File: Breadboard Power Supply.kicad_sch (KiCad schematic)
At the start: 15 parts, among them J1 Conn_01x02, J2 Conn_01x02, J3 Conn_01x03, J4 Screw_Terminal_01x02, J5 Barrel_Jack, U1 LM7805_TO220, U2 LM317_TO-220

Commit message: footprints
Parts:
- C1, C2, C3: footprint (none) -> Capacitor_THT:C_Disc_D3.0mm_W1.6mm_P2.50mm
- D1: footprint (none) -> LED_THT:LED_D5.0mm
- J1, J2: footprint (none) -> Connector_PinHeader_2.54mm:PinHeader_1x02_P2.54mm_Vertical
- J3: footprint (none) -> Connector_PinHeader_2.54mm:PinHeader_1x03_P2.54mm_Vertical
- J4: footprint (none) -> TerminalBlock:TerminalBlock_bornier-2_P5.08mm
- J5: footprint (none) -> Connector_BarrelJack:BarrelJack_SwitchcraftConxall_RAPC10U_Horizontal
- R1, R2, R3: footprint (none) -> PCM_Resistor_THT_AKL:R_Axial_DIN0204_L3.6mm_D1.6mm_P7.62mm_Horizontal
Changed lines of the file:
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@@
 			)
 		)
-		(property "Footprint" ""
+		(property "Footprint" "Capacitor_THT:C_Disc_D3.0mm_W1.6mm_P2.50mm"
 			(at 87.3252 66.04 0)
 			(effects
@@
 			)
 		)
-		(property "Footprint" ""
+		(property "Footprint" "PCM_Resistor_THT_AKL:R_Axial_DIN0204_L3.6mm_D1.6mm_P7.62mm_Horizontal"
 			(at 66.04 55.118 90)
 			(effects
@@
 			)
 		)
-		(property "Footprint" ""
+		(property "Footprint" "LED_THT:LED_D5.0mm"
 			(at 66.04 40.64 0)
 			(effects
@@
 			)
 		)
-		(property "Footprint" ""
+		(property "Footprint" "Capacitor_THT:C_Disc_D3.0mm_W1.6mm_P2.50mm"
 			(at 67.0052 66.04 0)
 			(effects
@@
 			)
 		)
-		(property "Footprint" ""
+		(property "Footprint" "Connector_PinHeader_2.54mm:PinHeader_1x02_P2.54mm_Vertical"
 			(at 66.04 72.39 0)
 			(effects
@@
 			)
 		)
-		(property "Footprint" ""
+		(property "Footprint" "TerminalBlock:TerminalBlock_bornier-2_P5.08mm"
 			(at 90.17 82.55 0)
 			(effects
@@
 			)
 		)
-		(property "Footprint" ""
+		(property "Footprint" "PCM_Resistor_THT_AKL:R_Axial_DIN0204_L3.6mm_D1.6mm_P7.62mm_Horizontal"
 			(at 86.36 55.118 90)
 			(effects
@@
 			)
 		)
-		(property "Footprint" ""
+		(property "Footprint" "PCM_Resistor_THT_AKL:R_Axial_DIN0204_L3.6mm_D1.6mm_P7.62mm_Horizontal"
 			(at 76.2 55.118 90)
 			(effects
@@
 			)
 		)
-		(property "Footprint" ""
+		(property "Footprint" "Connector_BarrelJack:BarrelJack_SwitchcraftConxall_RAPC10U_Horizontal"
 			(at 67.31 26.416 0)
 			(effects
@@
 			)
 		)
-		(property "Footprint" ""
+		(property "Footprint" "Connector_PinHeader_2.54mm:PinHeader_1x02_P2.54mm_Vertical"
 			(at 86.36 72.39 0)
 			(effects
@@
 			)
 		)
-		(property "Footprint" ""
+		(property "Footprint" "Connector_PinHeader_2.54mm:PinHeader_1x03_P2.54mm_Vertical"
 			(at 67.31 83.82 0)
 			(effects
@@
 			)
 		)
-		(property "Footprint" ""
+		(property "Footprint" "Capacitor_THT:C_Disc_D3.0mm_W1.6mm_P2.50mm"
 			(at 77.1652 66.04 0)
 			(effects

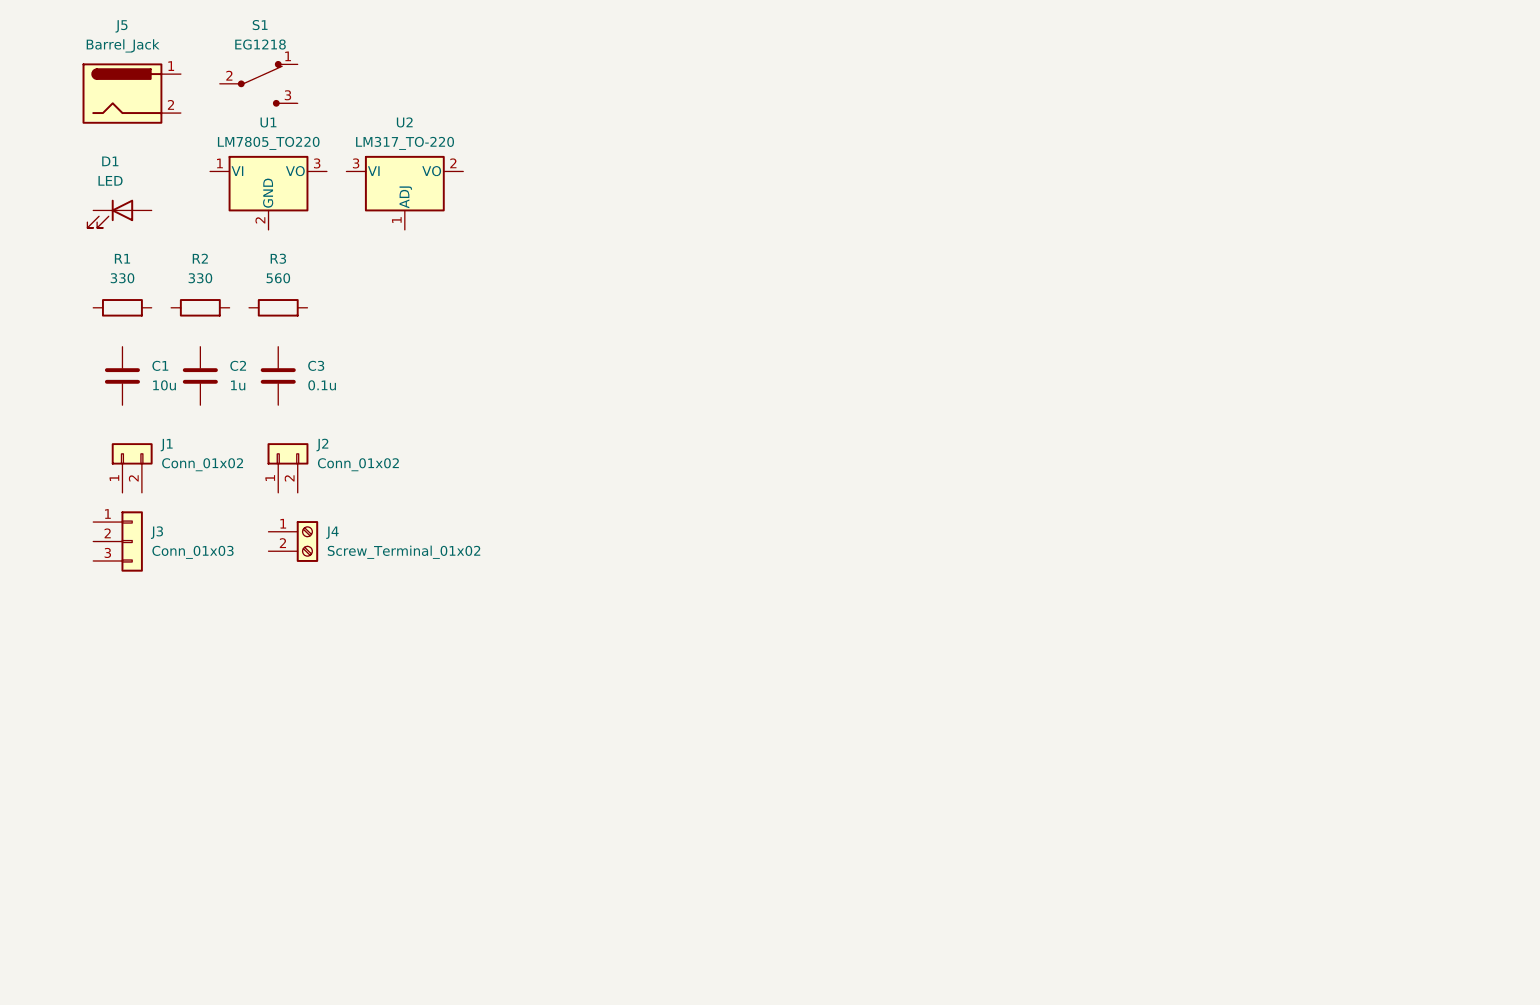
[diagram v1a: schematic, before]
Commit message: schematic + placing
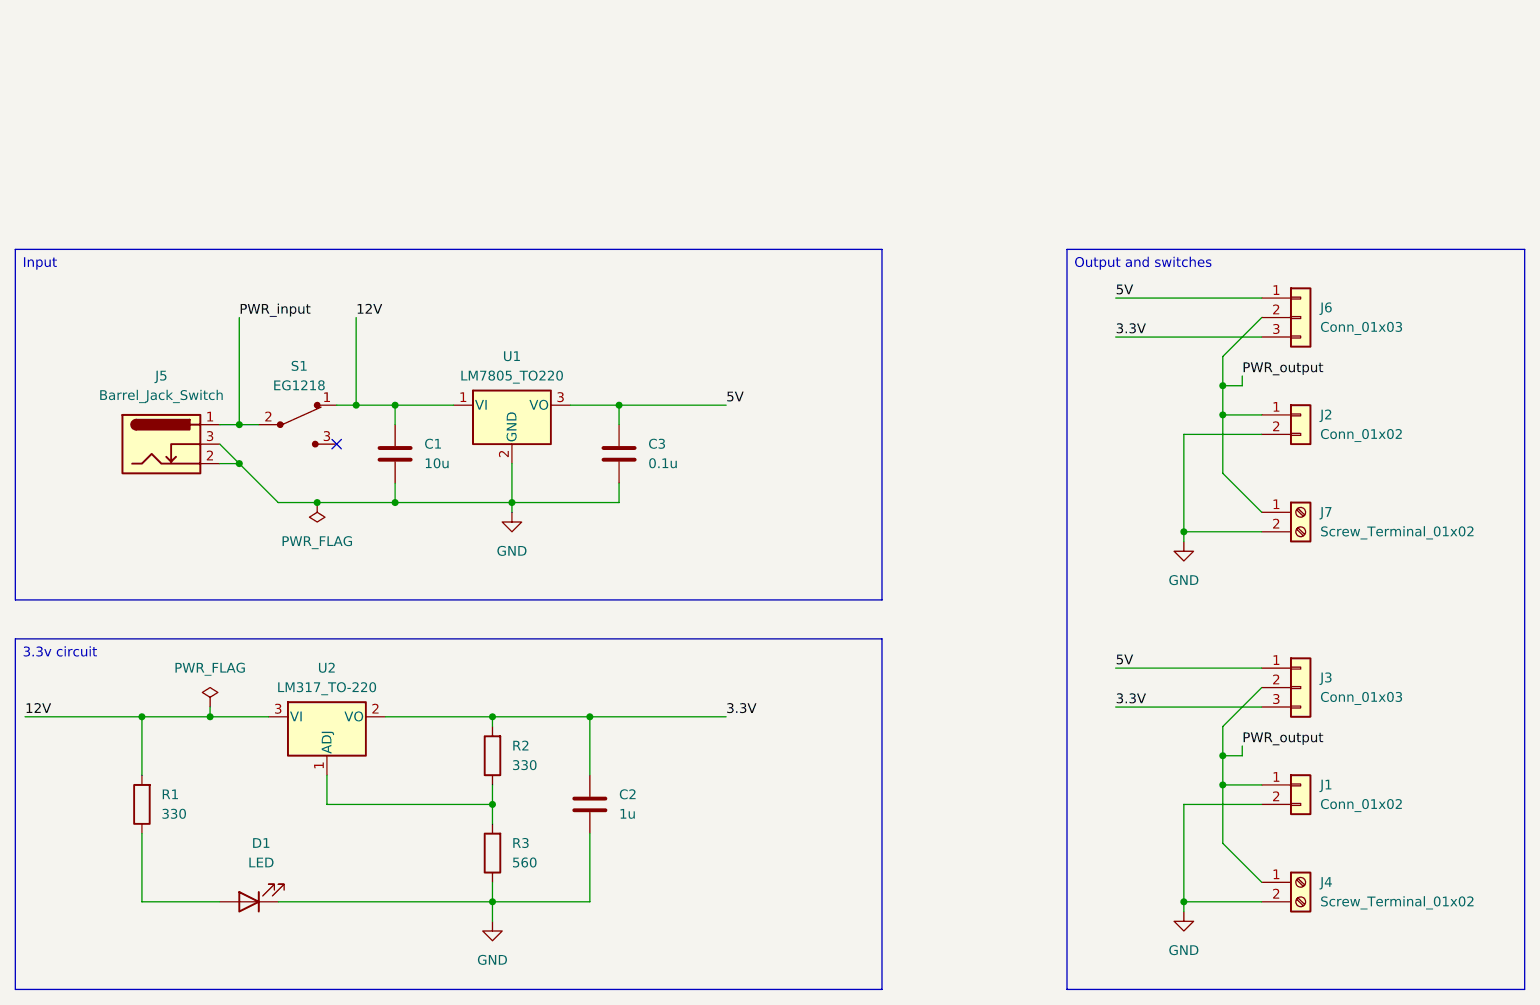
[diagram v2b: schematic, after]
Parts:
- removed J5: Barrel_Jack, Connector_BarrelJack:BarrelJack_SwitchcraftConxall_RAPC10U_Horizontal, symbol Connector:Barrel_Jack
- added J5: Barrel_Jack_Switch, Connector_BarrelJack:BarrelJack_Horizontal, symbol Connector:Barrel_Jack_Switch
- added J6: Conn_01x03, Connector_PinHeader_2.54mm:PinHeader_1x03_P2.54mm_Vertical, symbol Connector_Generic:Conn_01x03
- added J7: Screw_Terminal_01x02, TerminalBlock:TerminalBlock_bornier-2_P5.08mm, symbol Connector:Screw_Terminal_01x02
- D1: footprint LED_THT:LED_D5.0mm -> (none)
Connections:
- net 12V: now reaches S1.1
- net 12V: now also C1.1, R1.2, U1.1 (VI), U2.3 (VI)
- net PWR_input: now reaches S1.2
- net PWR_input: now also J5.1
- net 5V: now reaches C3.1
- net 5V: now also J3.1 (Pin_1), U1.3 (VO), J6.1 (Pin_1)
- net GND: now reaches C3.2
- net GND: now also C1.2, C2.2, D1.1 (K), J1.2 (Pin_2), J2.2 (Pin_2), J4.2 (Pin_2), R3.1, U1.2 (GND), J5.2, J5.3, J7.2 (Pin_2)
- net at R1.1: now also D1.2 (A)
- net PWR_output: now reaches J1.1 (Pin_1)
- net PWR_output: now also J2.1 (Pin_1), J3.2 (Pin_2), J4.1 (Pin_1), J6.2 (Pin_2), J7.1 (Pin_1)
- net at U2.1 (ADJ): now also R2.1, R3.2
- net 3.3V: now reaches U2.2 (VO)
- net 3.3V: now also C2.1, J3.3 (Pin_3), R2.2, J6.3 (Pin_3)
- no-connect marks 0 -> 1
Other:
- moved on the sheet: C1, C2, C3, J1, J3, J4, R1, R2, R3, S1, U1, U2
